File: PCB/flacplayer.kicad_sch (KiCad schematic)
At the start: 85 parts, among them J1 Micro_SD_Card_Det_Hirose_DM3AT, J2 USB_C_Receptacle_USB2.0, J4 Conn_01x24_MountingPin, J5 AudioJack3, Q1 PMOS, Q2 AO3400A, Q3 AO3401A, Q4 NMOS, SW1 SW_Push, SW2 SW_Push, SW3 SW_Push, SW4 SW_Push, SW5 SW_Push, SW6 SW_Push, SW7 SW_Push, U1 ESP32-S3-MINI-1, U2 MAX17048X, U3 AMS1117-3.3, U5 TAD5242, U6 TPA6132A2RTE, U7 MCP73831-2-OT

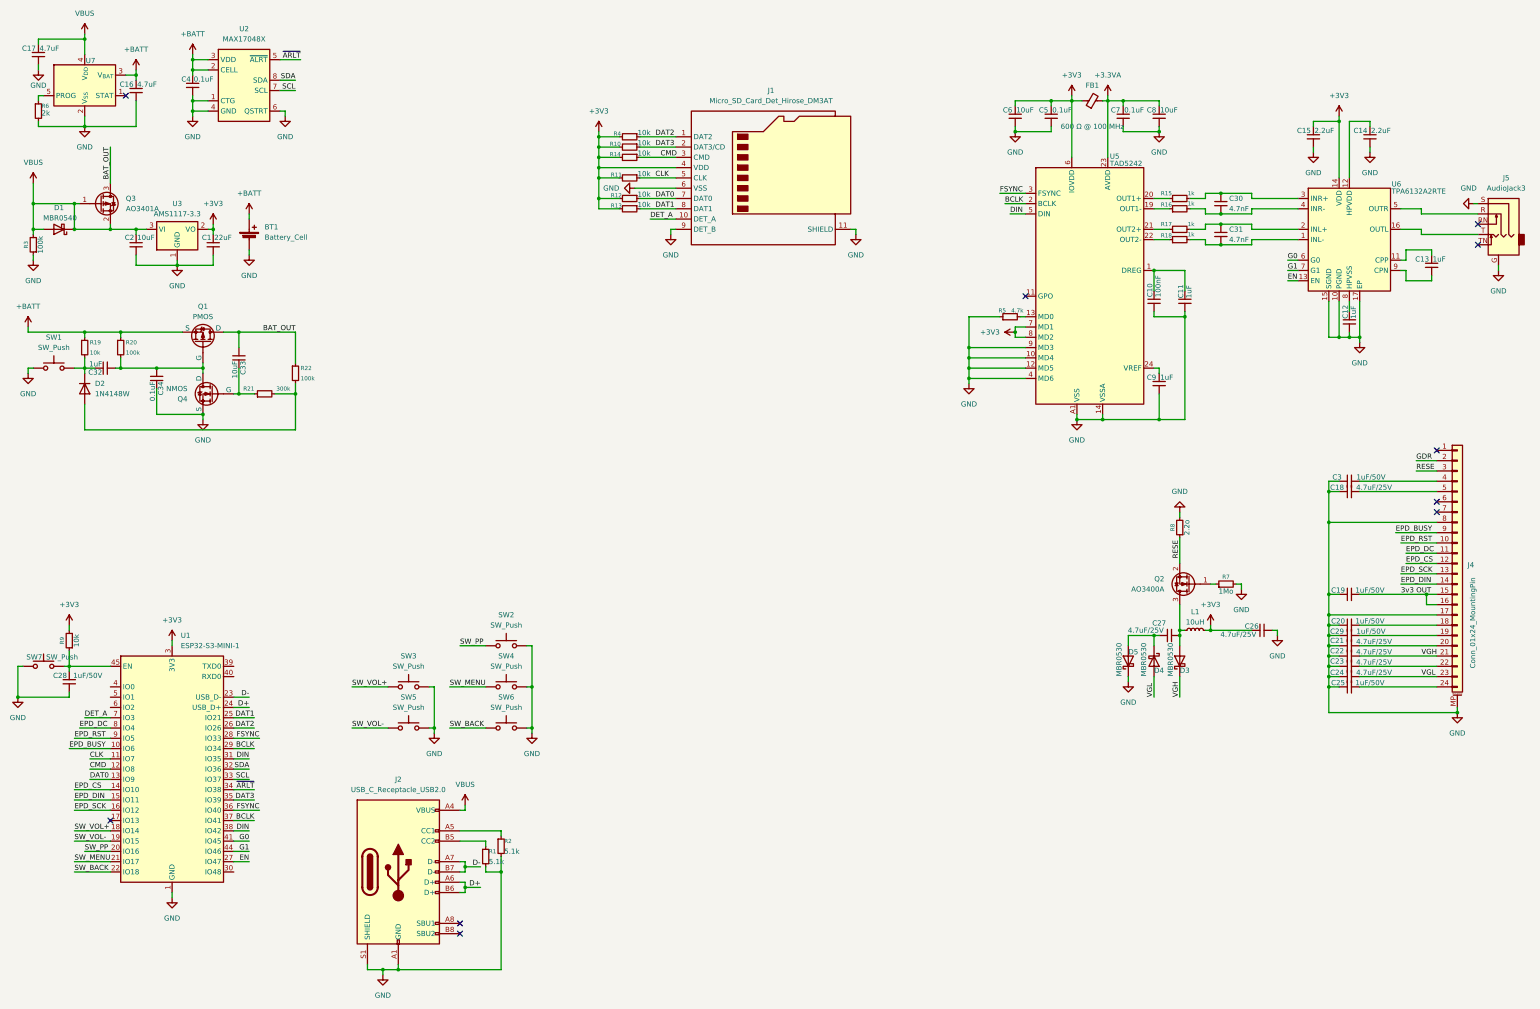
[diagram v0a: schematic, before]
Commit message: NEW journal weeeeeeeee i talk about remaking it beh
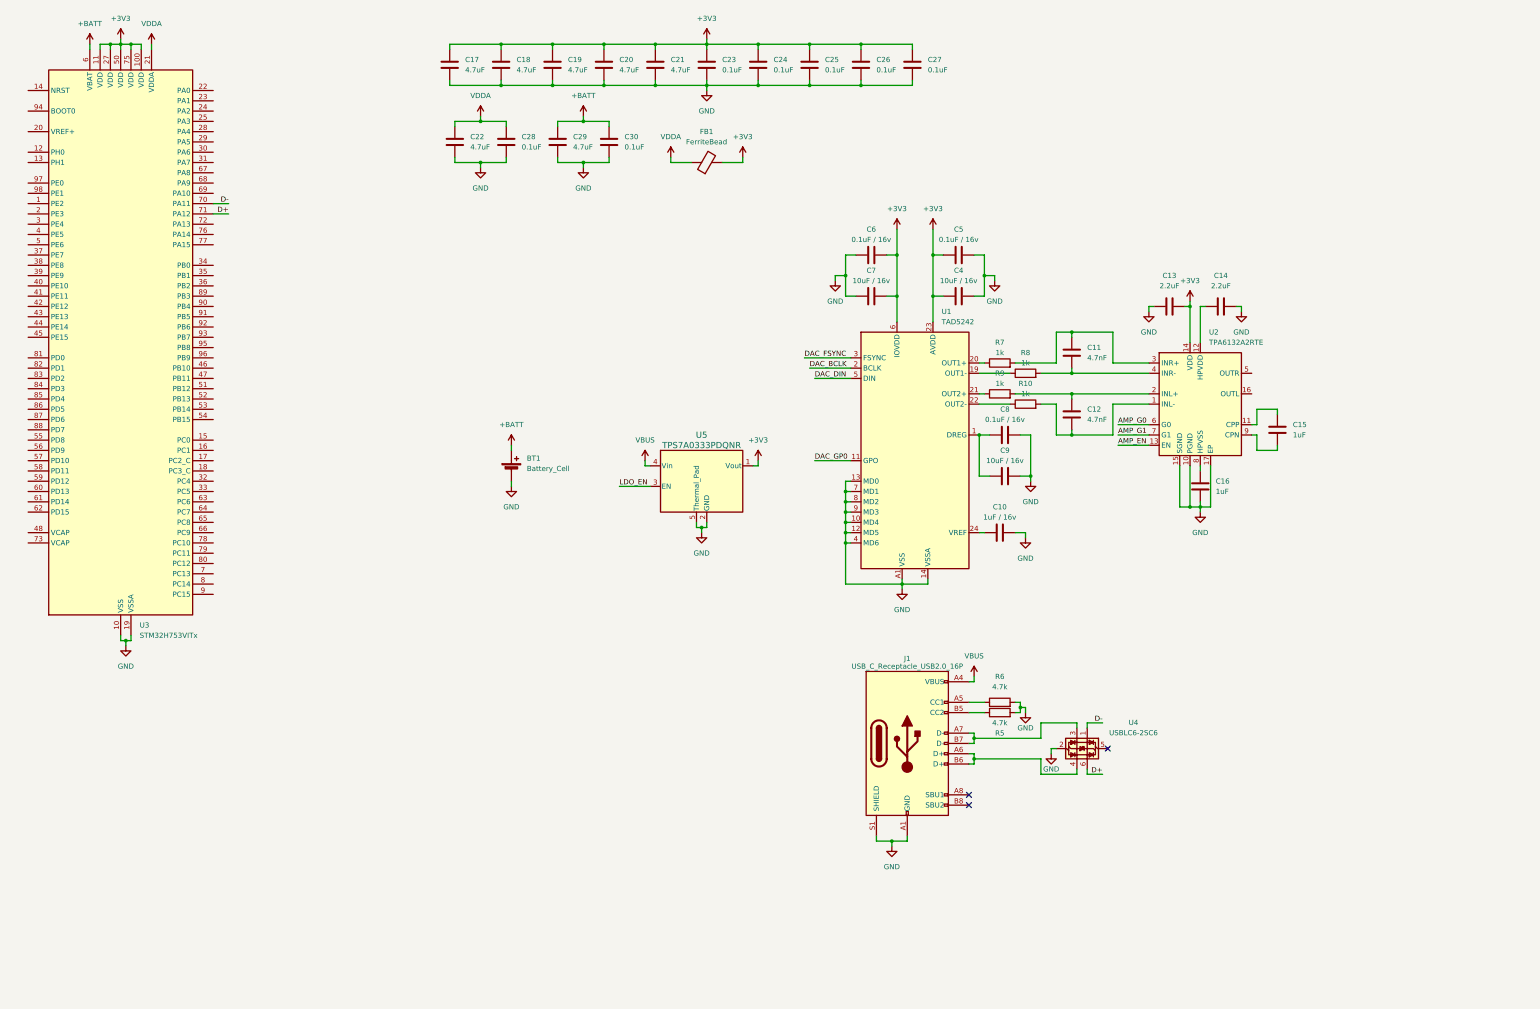
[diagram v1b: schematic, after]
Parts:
- removed C1: 22uF, Capacitor_SMD:C_0603_1608Metric_Pad1.08x0.95mm_HandSolder, symbol Device:C_Small
- removed C10: 100nF, Capacitor_SMD:C_0603_1608Metric_Pad1.08x0.95mm_HandSolder, symbol Device:C_Small
- removed C11, C12, C13, C32, C9: 1uF, Capacitor_SMD:C_0603_1608Metric_Pad1.08x0.95mm_HandSolder, symbol Device:C_Small
- removed C14, C15: 2.2uF, Capacitor_SMD:C_0603_1608Metric_Pad1.08x0.95mm_HandSolder, symbol Device:C_Small
- removed C16, C17: 4.7uF, Capacitor_SMD:C_0603_1608Metric_Pad1.08x0.95mm_HandSolder, symbol Device:C_Small
- removed C18, C21, C22, C23, C24, C26, C27: 4.7uF/25V, Capacitor_SMD:C_0603_1608Metric_Pad1.08x0.95mm_HandSolder, symbol Device:C_Small
- removed C19, C20, C25, C28, C29, C3: 1uF/50V, Capacitor_SMD:C_0603_1608Metric_Pad1.08x0.95mm_HandSolder, symbol Device:C_Small
- removed C2, C33, C6, C8: 10uF, Capacitor_SMD:C_0603_1608Metric_Pad1.08x0.95mm_HandSolder, symbol Device:C_Small
- removed C30, C31: 4.7nF, Capacitor_SMD:C_0603_1608Metric_Pad1.08x0.95mm_HandSolder, symbol Device:C_Small
- removed C34, C4, C5, C7: 0.1uF, Capacitor_SMD:C_0603_1608Metric_Pad1.08x0.95mm_HandSolder, symbol Device:C_Small
- removed D1: MBR0540, Diode_SMD:D_SOD-123, symbol Diode:MBR0540
- removed D2: 1N4148W, Diode_SMD:D_SOD-123, symbol Diode:1N4148W
- removed D3, D4, D5: MBR0530, Diode_SMD:D_SOD-123, symbol Diode:MBR0530
- removed FB1: 600 Ω @ 100 MHz, footprints:FB_0603, symbol Device:FerriteBead_Small
- removed J1: Micro_SD_Card_Det_Hirose_DM3AT, Connector_Card:microSD_HC_Hirose_DM3AT-SF-PEJM5, symbol Connector:Micro_SD_Card_Det_Hirose_DM3AT
- removed J2: USB_C_Receptacle_USB2.0, Connector_USB:USB_C_Receptacle_HCTL_HC-TYPE-C-16P-01A, symbol Connector:USB_C_Receptacle_USB2.0_16P
- removed J4: Conn_01x24_MountingPin, Connector_FFC-FPC:Amphenol_F32R-1A7x1-11024_1x24-1MP_P0.5mm_Horizontal, symbol Connector_Generic_MountingPin:Conn_01x24_MountingPin
- removed J5: AudioJack3, footprints:SHOU-HAN-PJ-242, symbol Connector_Audio:AudioJack3_Ground_SwitchTR
- removed L1: 10uH, Inductor_SMD:L_0603_1608Metric, symbol Device:L_Small
- removed Q1: PMOS, symbol Simulation_SPICE:PMOS
- removed Q2: AO3400A, Package_TO_SOT_SMD:SOT-23, symbol Transistor_FET:AO3400A
- removed Q3: AO3401A, Package_TO_SOT_SMD:SOT-23, symbol Transistor_FET:AO3401A
- removed Q4: NMOS, symbol Simulation_SPICE:NMOS
- removed R1, R2: 5.1k, Resistor_SMD:R_0603_1608Metric, symbol Device:R_Small
- removed R10, R11, R12, R13, R14, R4, R9: 10k, Resistor_SMD:R_0603_1608Metric, symbol Device:R_Small
- removed R15, R16, R17, R18: 1k, Resistor_SMD:R_0603_1608Metric, symbol Device:R_Small
- removed R19: 10k, symbol Device:R_Small
- removed R20, R22: 100k, symbol Device:R_Small
- removed R21: 300k, symbol Device:R_Small
- removed R3: 100k, Resistor_SMD:R_0603_1608Metric, symbol Device:R_Small
- removed R5: 4.7k, Resistor_SMD:R_0603_1608Metric, symbol Device:R_Small
- removed R6: 2k, Resistor_SMD:R_0603_1608Metric, symbol Device:R_Small
- removed R7: 1Mo, Resistor_SMD:R_0603_1608Metric, symbol Device:R_Small
- removed R8: 2.2o, Resistor_SMD:R_0603_1608Metric, symbol Device:R_Small
- removed SW1, SW2, SW3, SW4, SW5, SW6, SW7: SW_Push, symbol Switch:SW_Push
- removed U1: ESP32-S3-MINI-1, RF_Module:ESP32-S2-MINI-1, symbol RF_Module:ESP32-S3-MINI-1
- removed U2: MAX17048X, smth:WLP-8_1.67x0.93_P0.4, symbol ultraflat-lib:MAX17048X
- removed U3: AMS1117-3.3, Package_TO_SOT_SMD:SOT-223-3_TabPin2, symbol Regulator_Linear:AMS1117-3.3
- removed U5: TAD5242, footprints:Texas_RGE0024R_VQFN-24-1EP_4x4mm_P0.5mm_EP2.1x2.1mm, symbol TAD5242:TAD5242
- removed U6: TPA6132A2RTE, Package_DFN_QFN:WQFN-16-1EP_3x3mm_P0.5mm_EP1.6x1.6mm_ThermalVias, symbol Amplifier_Audio:TPA6132A2RTE
- removed U7: MCP73831-2-OT, Package_TO_SOT_SMD:SOT-23-5, symbol Battery_Management:MCP73831-2-OT
- added C10: 1uF / 16v, symbol Device:C
- added C11, C12: 4.7nF, symbol Device:C
- added C13, C14: 2.2uF, symbol Device:C
- added C15, C16: 1uF, symbol Device:C
- added C17, C18, C19, C20, C21, C22, C29: 4.7uF, symbol Device:C
- added C23, C24, C25, C26, C27, C28, C30: 0.1uF, symbol Device:C
- added C4, C7, C9: 10uF / 16v, symbol Device:C
- added C5, C6, C8: 0.1uF / 16v, symbol Device:C
- added FB1: FerriteBead, symbol Device:FerriteBead
- added J1: USB_C_Receptacle_USB2.0_16P, symbol Connector:USB_C_Receptacle_USB2.0_16P
- added R10, R7, R8, R9: 1k, symbol Device:R
- added R5, R6: 4.7k, symbol Device:R
- added U1: TAD5242, footprints:Texas_RGE0024R_VQFN-24-1EP_4x4mm_P0.5mm_EP2.1x2.1mm, symbol TAD5242:TAD5242
- added U2: TPA6132A2RTE, Package_DFN_QFN:WQFN-16-1EP_3x3mm_P0.5mm_EP1.6x1.6mm_ThermalVias, symbol Amplifier_Audio:TPA6132A2RTE
- added U3: STM32H753VITx, Package_QFP:LQFP-100_14x14mm_P0.5mm, symbol MCU_ST_STM32H7:STM32H753VITx
- added U4: USBLC6-2SC6, Package_TO_SOT_SMD:SOT-23-6, symbol Power_Protection:USBLC6-2SC6
- added U5: TPS7A0333PDQNR, DQN0004A-MFG, symbol 2026-06-11_14-57-08:TPS7A0333PDQNR
- BT1: footprint Connector_PinHeader_2.54mm:PinHeader_1x02_P2.54mm_Vertical -> (none)
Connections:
- net +3V3: now also C13.2, C17.1, C18.1, C19.1, C20.1, C21.1, C23.1, C24.1, C25.1, C26.1, C27.1, C4.1, C5.1, C6.2, C7.2, FB1.2, U1.23 (AVDD), U1.6 (IOVDD), U2.14 (VDD), U3.100 (VDD), U3.11 (VDD), U3.27 (VDD), U3.50 (VDD), U3.75 (VDD), U5.1 (Vout)
- net +BATT: now also C29.1, C30.1, U3.6 (VBAT)
- net D+: now also U3.71 (PA12), U4.6 (I/O1)
- net D-: now also U3.70 (PA11), U4.1 (I/O1)
- net GND: now also C10.2, C13.1, C14.2, C16.2, C17.2, C18.2, C19.2, C20.2, C21.2, C22.2, C23.2, C24.2, C25.2, C26.2, C27.2, C28.2, C29.2, C30.2, C4.2, C5.2, C6.1, C7.1, C8.2, C9.2, J1.A1 (GND), J1.A12 (GND), J1.B1 (GND), J1.B12 (GND), J1.S1 (SHIELD), R5.2, R6.2, U1.10 (MD4), U1.12 (MD5), U1.13 (MD0), U1.14 (VSSA), U1.15 (VSSA), U1.16 (VSSA), U1.17 (VSSA), U1.18 (VSSA), U1.25 (VSS), U1.4 (MD6), U1.7 (MD1), U1.8 (MD2), U1.9 (MD3), U1.A1 (VSS), U1.A2 (VSS), U1.A3 (VSS), U1.A4 (VSS), U2.10 (PGND), U2.15 (SGND), U2.17 (EP), U3.10 (VSS), U3.19 (VSSA), U3.26 (VSS), U3.49 (VSS), U3.74 (VSS), U3.99 (VSS), U4.2 (GND), U5.2 (GND), U5.5 (Thermal_Pad)
- net VBUS: now also J1.A4 (VBUS), J1.A9 (VBUS), J1.B4 (VBUS), J1.B9 (VBUS), U5.4 (Vin)
- new net: R10.1, U1.22 (OUT2-)
- new net: C12.2, R10.2, U2.1 (INL-)
- new net: J1.A7 (D-), J1.B7 (D-), U4.3 (I/O2)
- new net: J1.A6 (D+), J1.B6 (D+), U4.4 (I/O2)
- new net: C11.1, R7.2, U2.3 (INR+)
- new net: C11.2, R8.2, U2.4 (INR-)
- new net: R7.1, U1.20 (OUT1+)
- new net: C16.1, U2.8 (HPVSS)
- new net: R8.1, U1.19 (OUT1-)
- new net: C15.1, U2.11 (CPP)
- new net: C14.1, U2.12 (HPVDD)
- new net: C12.1, R9.2, U2.2 (INL+)
- new net: C15.2, U2.9 (CPN)
- new net: J1.A5 (CC1), R6.1
- new net: J1.B5 (CC2), R5.1
- new net: C8.1, C9.1, U1.1 (DREG)
- new net: R9.1, U1.21 (OUT2+)
- new net: C10.1, U1.24 (VREF)
- new net AMP_EN: U2.13 (EN)
- new net AMP_G0: U2.6 (G0)
- new net AMP_G1: U2.7 (G1)
- new net DAC_BCLK: U1.2 (BCLK)
- new net DAC_DIN: U1.5 (DIN)
- new net DAC_FSYNC: U1.3 (FSYNC)
- new net DAC_GP0: U1.11 (GPO)
- new net LDO_EN: U5.3 (EN)
- new net VDDA: C22.1, C28.1, FB1.1, U3.21 (VDDA)
- no-connect marks 10 -> 3

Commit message: mpu6050 ayya accel and gyro + journal
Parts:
- added C1: 2.2nF, 50V, symbol Device:C
- added C2: 0.1μF, 2V, symbol Device:C
- added C3: 10nF, 4V, symbol Device:C
- added C31: 0.1μF, 4V, symbol Device:C
- added J2: AudioJack4, symbol Connector_Audio:AudioJack4
- added U6: MPU-6050, Sensor_Motion:InvenSense_QFN-24_4x4mm_P0.5mm, symbol Sensor_Motion:MPU-6050
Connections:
- net +3V3: now also C3.1, C31.1, U6.13 (VDD), U6.8 (VLOGIC)
- net GND: now also C1.2, C2.2, C3.2, C31.2, J2.R2, U6.18 (GND)
- net at U2.16 (OUTL): now also J2.T
- net at U2.5 (OUTR): now also J2.R1
- new net: C2.1, U6.10 (REGOUT)
- new net: C1.1, U6.20 (CPOUT)
- new net MPU_AD0: U6.9 (AD0)
- new net MPU_INT: U6.12 (INT)
- new net MPU_SCL: U6.23 (SCL)
- new net MPU_SDA: U6.24 (SDA)
- no-connect marks 3 -> 8
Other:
- moved on the sheet: BT1, C10, C11, C12, C13, C14, C15, C16, C17, C18, C19, C20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

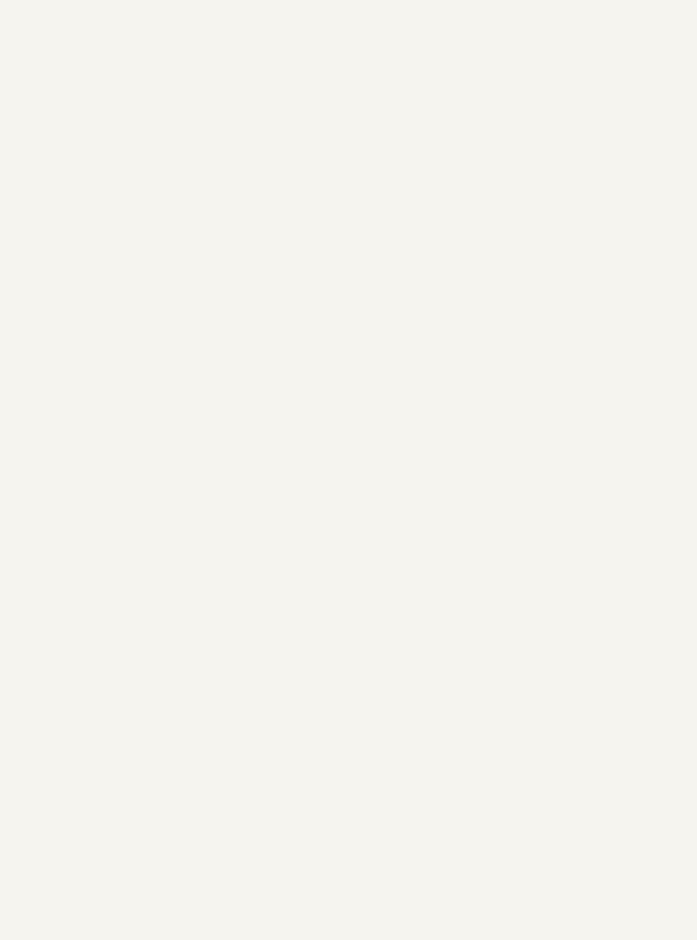
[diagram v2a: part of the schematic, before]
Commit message: epaper
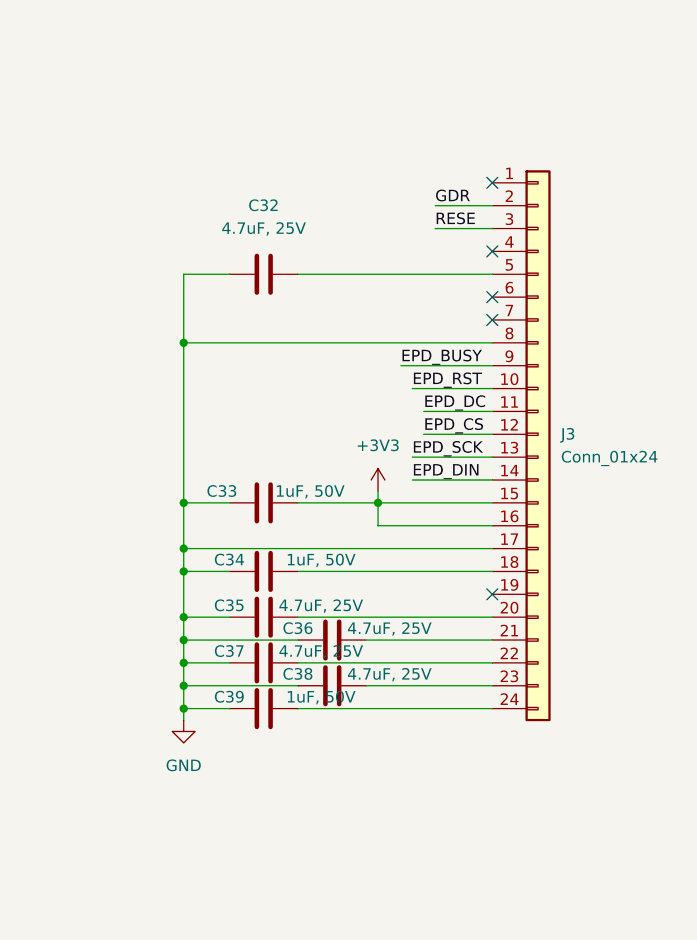
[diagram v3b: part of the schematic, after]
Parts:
- added C32, C35, C36, C37, C38: 4.7uF, 25V, symbol Device:C
- added C33, C34, C39: 1uF, 50V, symbol Device:C
- added J3: Conn_01x24, symbol Connector_Generic:Conn_01x24
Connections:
- net +3V3: now also C33.2, J3.15 (Pin_15), J3.16 (Pin_16)
- net GND: now also C32.1, C33.1, C34.1, C35.1, C36.1, C37.1, C38.1, C39.1, J3.17 (Pin_17), J3.8 (Pin_8)
- new net: C36.2, J3.21 (Pin_21)
- new net: C34.2, J3.18 (Pin_18)
- new net: C35.2, J3.20 (Pin_20)
- new net: C37.2, J3.22 (Pin_22)
- new net: C38.2, J3.23 (Pin_23)
- new net: C39.2, J3.24 (Pin_24)
- new net: C32.2, J3.5 (Pin_5)
- new net EPD_BUSY: J3.9 (Pin_9)
- new net EPD_CS: J3.12 (Pin_12)
- new net EPD_DC: J3.11 (Pin_11)
- new net EPD_DIN: J3.14 (Pin_14)
- new net EPD_RST: J3.10 (Pin_10)
- new net EPD_SCK: J3.13 (Pin_13)
- new net GDR: J3.2 (Pin_2)
- new net RESE: J3.3 (Pin_3)
- no-connect marks 8 -> 13
